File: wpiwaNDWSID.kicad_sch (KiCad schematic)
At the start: 14 parts, among them J1 USB_C_Receptacle_USB2.0_16P, J2 Conn_01x02, J3 Conn_01x04, U1 AP63205WU, U2 AP7363-33D-13

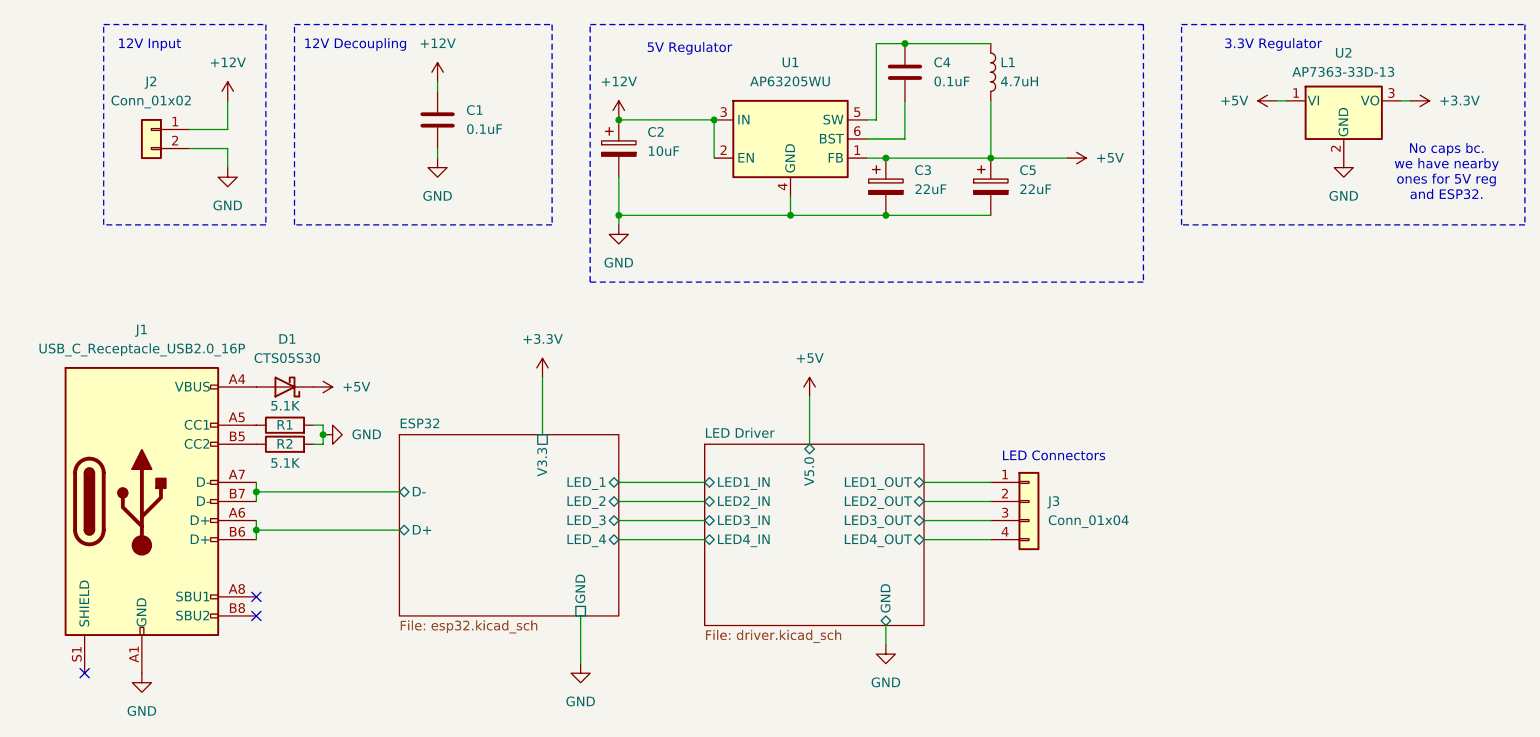
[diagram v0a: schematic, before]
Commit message: rev 2
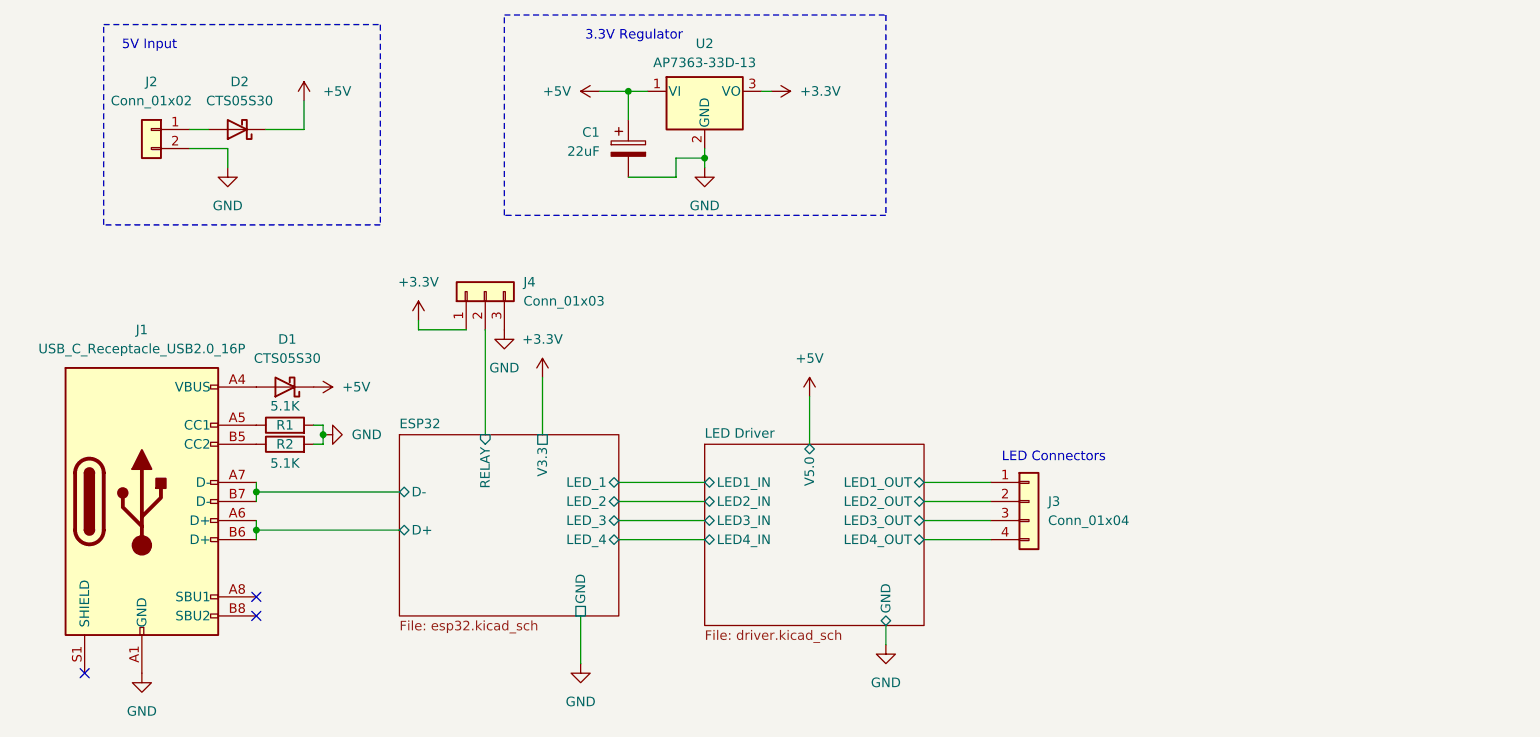
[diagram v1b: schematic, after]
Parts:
- removed C1, C4: 0.1uF, Capacitor_SMD:C_0402_1005Metric, symbol Device:C
- removed C2: 10uF, Capacitor_THT:CP_Radial_D4.0mm_P2.00mm, symbol Device:C_Polarized
- removed C3, C5: 22uF, Capacitor_THT:CP_Radial_D4.0mm_P2.00mm, symbol Device:C_Polarized
- removed L1: 4.7uH, Inductor_SMD:L_0603_1608Metric_Pad1.05x0.95mm_HandSolder, symbol Device:L
- removed U1: AP63205WU, Package_TO_SOT_SMD:TSOT-23-6_HandSoldering, symbol Regulator_Switching:AP63205WU
- added C1: 22uF, Capacitor_THT:CP_Radial_D4.0mm_P2.00mm, symbol Device:C_Polarized
- added D2: CTS05S30, Diode_SMD:D_0402_1005Metric_Pad0.77x0.64mm_HandSolder, symbol Diode:B220
- added J4: Conn_01x03, Connector_Wire:SolderWire-0.75sqmm_1x03_P4.8mm_D1.25mm_OD2.3mm, symbol Connector_Generic:Conn_01x03
- D1: footprint Diode_SMD:D_0805_2012Metric -> Diode_SMD:D_0402_1005Metric_Pad0.77x0.64mm_HandSolder
- J2: footprint Connector_Wire:SolderWire-1.5sqmm_1x02_P7.8mm_D1.7mm_OD3.9mm -> Connector_Wire:SolderWire-0.75sqmm_1x02_P4.8mm_D1.25mm_OD2.3mm
- J3: footprint Connector_Wire:SolderWire-1.5sqmm_1x04_P7.8mm_D1.7mm_OD3.9mm -> Connector_Wire:SolderWire-0.75sqmm_1x04_P4.8mm_D1.25mm_OD2.3mm
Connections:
- net +3.3V: now also J4.1 (Pin_1)
- net +5V: now also C1.1, D2.1 (K)
- net GND: now also C1.2, J4.3 (Pin_3)
- net +12V: no longer names the net of J2.1 (Pin_1)
- net +12V: now also D2.2 (A)
- new net ESP32/RELAY: J4.2 (Pin_2)
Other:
- sheet ESP32 ports: added RELAY; removed none
- note added: "5V Input"
- note removed: "12V Decoupling"
- note removed: "12V Input"
- note removed: "5V Regulator"
- note removed: "No caps bc. we have nearby ones for 5V reg and ESP32."
- moved on the sheet: U2
